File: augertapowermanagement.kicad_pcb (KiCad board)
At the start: 4 copper layers, 315.8 x 183 mm, 82 parts, among them J1 Screw_Terminal_01x02, J10 Screw_Terminal_01x10, J11 Screw_Terminal_01x10, J12 gnd block, J2 76825-0002, J3 USB_A_Stacked, J4 USB_A_Stacked, J5 USB_A_Stacked, J6 USB_A_Stacked, J7 Screw_Terminal_01x08, J8 Screw_Terminal_01x10, J9 5v block, K1 J107F1CS203VDC.80, K2 J107F1CS203VDC.80, SW1 SW_SPDT, U1 LM2596_5v, U10 INA219AxD, U11 INA219AxD, U12 LM2596_5v, U13 LM2596_5v, U14 INA219AxD, U15 INA219AxD, U16 LM2596_11.5v, U17 LM2596_5v, U18 INA219AxD, U19 INA219AxD, U2 ESP32-DEVKITC-32D, U20 LM2596_11.5v, U21 INA219AxD, U22 LM2596_11.5v, U23 INA219AxD, U24 MCP9808_MSOP, U3 INA219AxD, U4 LM2596_5v, U5 LM2596_5v, U6 INA219AxD, U7 INA219AxD, U8 LM2596_5v, U9 LM2596_5v

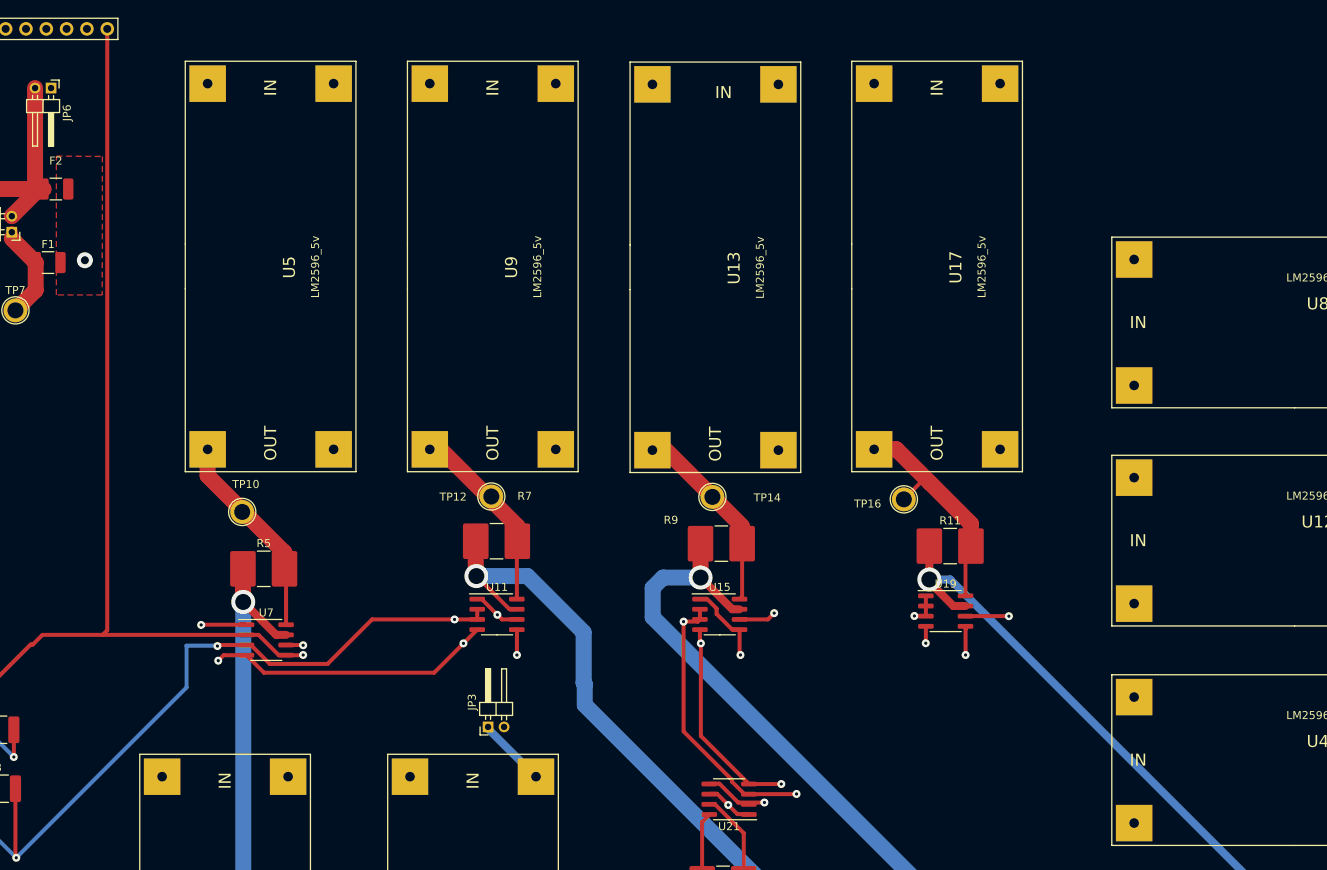
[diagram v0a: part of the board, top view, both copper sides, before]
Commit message: update
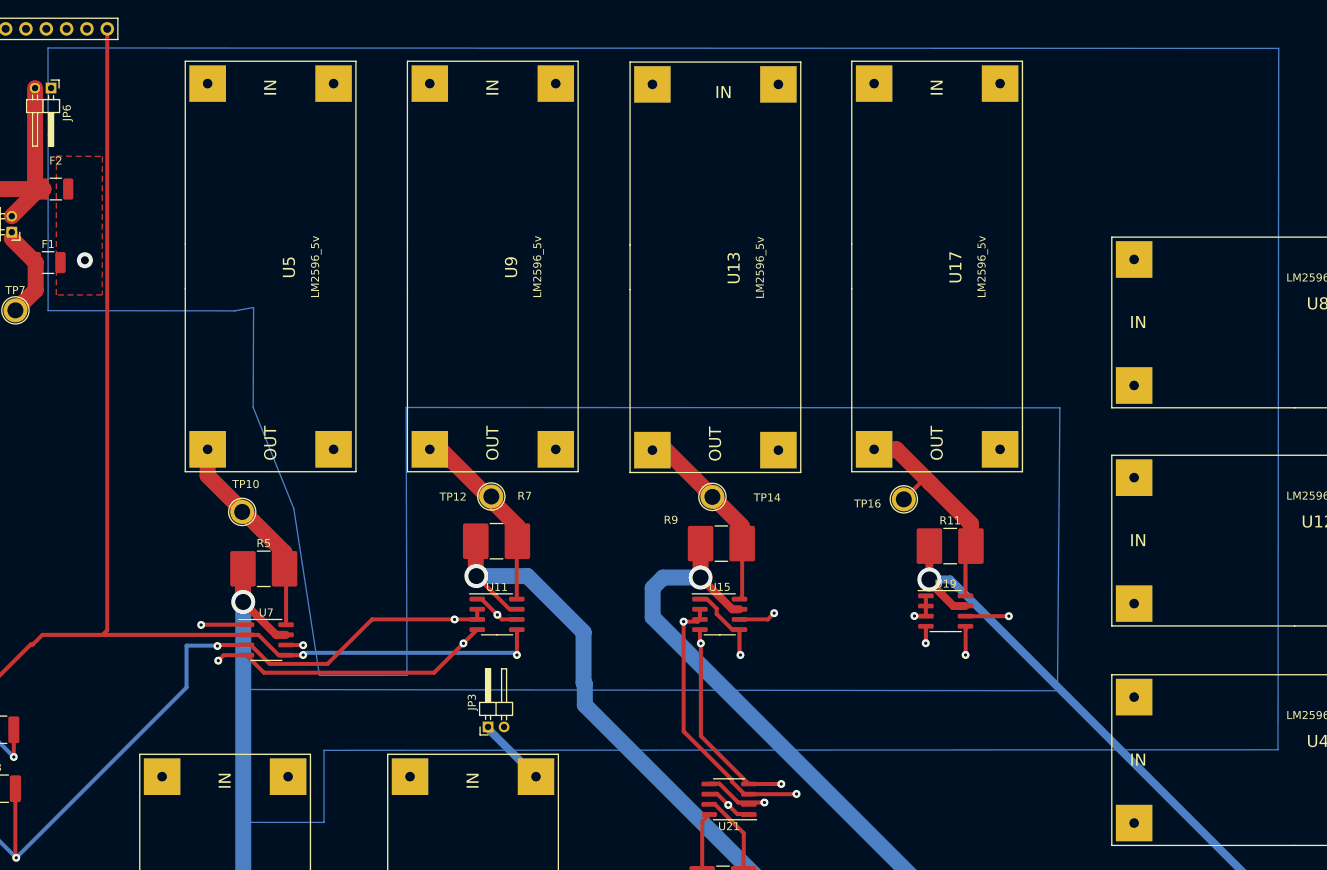
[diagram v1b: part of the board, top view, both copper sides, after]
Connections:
- J7 pad 1: unconnected-(J7-Pad1) -> /power_conversion/routerp
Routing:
- net /power_conversion/routerp: track 53.7 -> 72.3 mm
